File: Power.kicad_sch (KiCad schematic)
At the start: 17 parts, among them Q2 DNP, U25 LM66100DCK, U3 AZ1117CH-3.3TRG1, U4 LM66100DCK

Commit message: Before remove first clock input buffer
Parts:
- Q2: LCSC Part C20526 -> (none)
- R25, R26, R27: LCSC Part (none) -> C17798
- U25, U4: LCSC Part (none) -> C2869734
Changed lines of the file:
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@@
+			)
+		)
+		(property "LCSC Part" "C17798"
+			(at 128.27 105.41 0)
+			(effects
+				(font
+					(size 1.27 1.27)
+				)
+				(hide yes)
 			)
 		)
@@
 			)
 		)
+		(property "LCSC Part" "C2869734"
+			(at 100.33 86.36 0)
+			(effects
+				(font
+					(size 1.27 1.27)
+				)
+				(hide yes)
+			)
+		)
 		(pin "5"
 		)
@@
 			)
 		)
-		(property "LCSC Part" "C20526"
+		(property "LCSC Part" ""
 			(at 90.17 123.19 0)
 			(effects
@@
 			)
 		)
+		(property "LCSC Part" "C17798"
+			(at 148.59 105.41 0)
+			(effects
+				(font
+					(size 1.27 1.27)
+				)
+				(hide yes)
+			)
+		)
 		(pin "1"
 		)
@@
 			)
 		)
+		(property "LCSC Part" "C2869734"
+			(at 133.35 86.36 0)
+			(effects
+				(font
+					(size 1.27 1.27)
+				)
+				(hide yes)
+			)
+		)
 		(pin "5"
 		)
@@
 			(at 138.43 105.41 0)
 			(effects
+				(font
+					(size 1.27 1.27)
+				)
+				(hide yes)
+			)
+		)
+		(property "LCSC Part" "C17798"
+			(at 138.43 105.41 0)
+			(effects

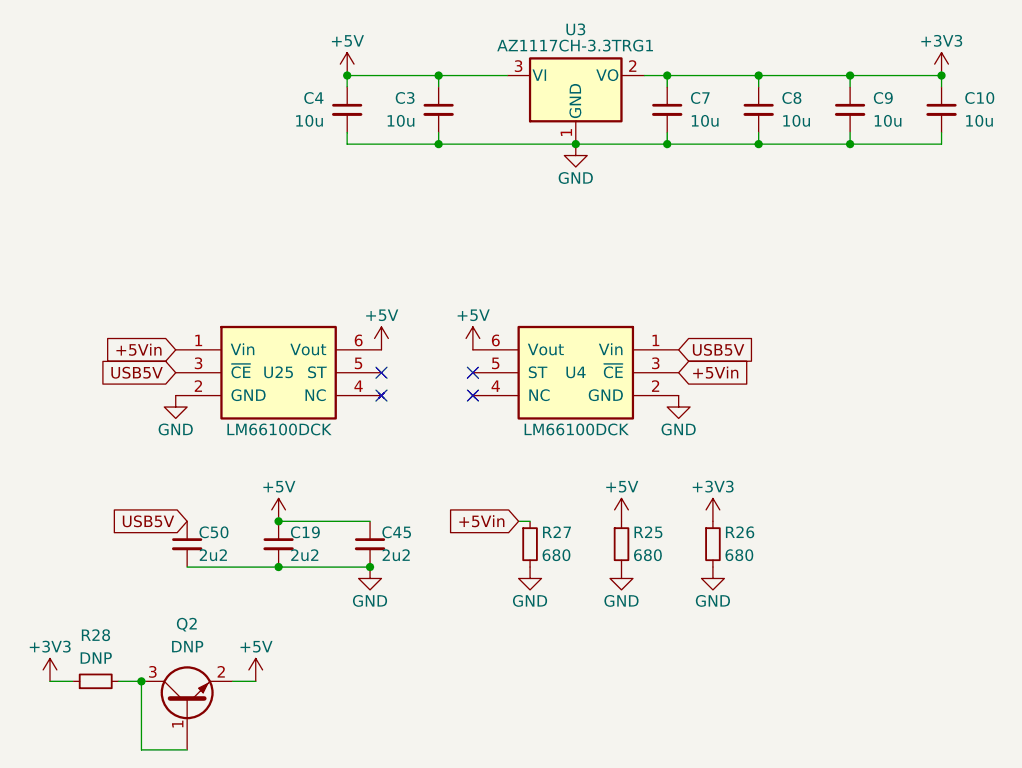
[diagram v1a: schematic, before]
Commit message: Final A?
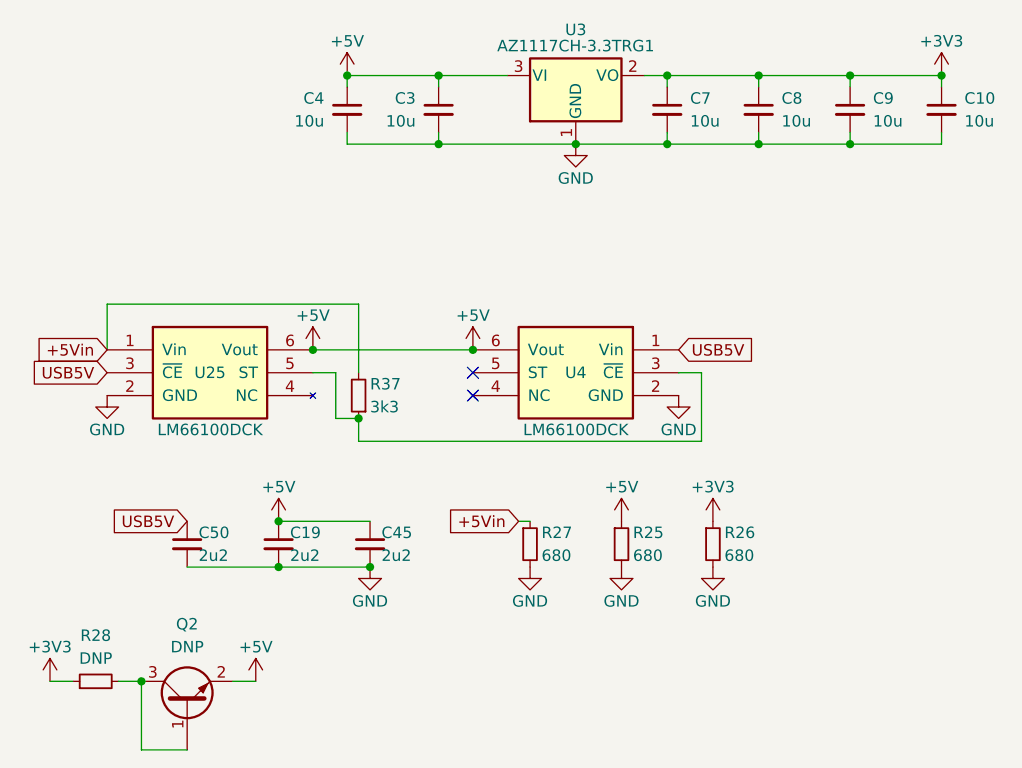
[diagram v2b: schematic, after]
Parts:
- added R37: 3k3, stdpads:R_0603, symbol Device:R_Small
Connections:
- net +5Vin: now also R37.2; no longer U4.3 (~{CE})
- net at U25.5 (ST): now also U4.3 (~{CE}), R37.1
- no-connect marks 4 -> 2
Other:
- moved on the sheet: U25
